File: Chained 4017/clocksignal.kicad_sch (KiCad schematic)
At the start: 6 parts, among them SW201 SW_Push, U201 LM555xM

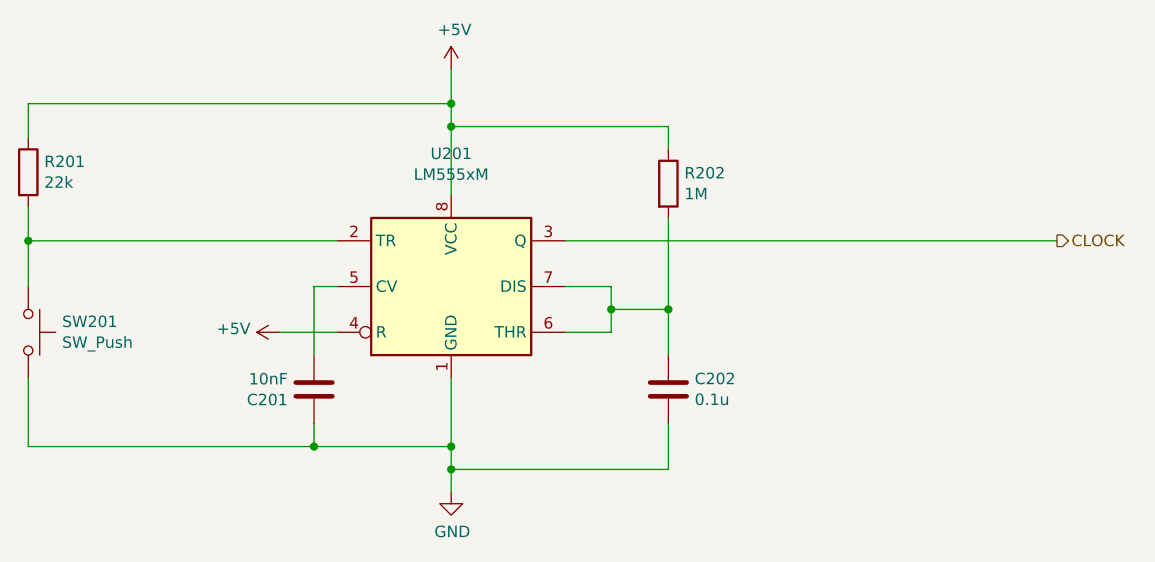
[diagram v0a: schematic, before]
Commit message: Complete routing
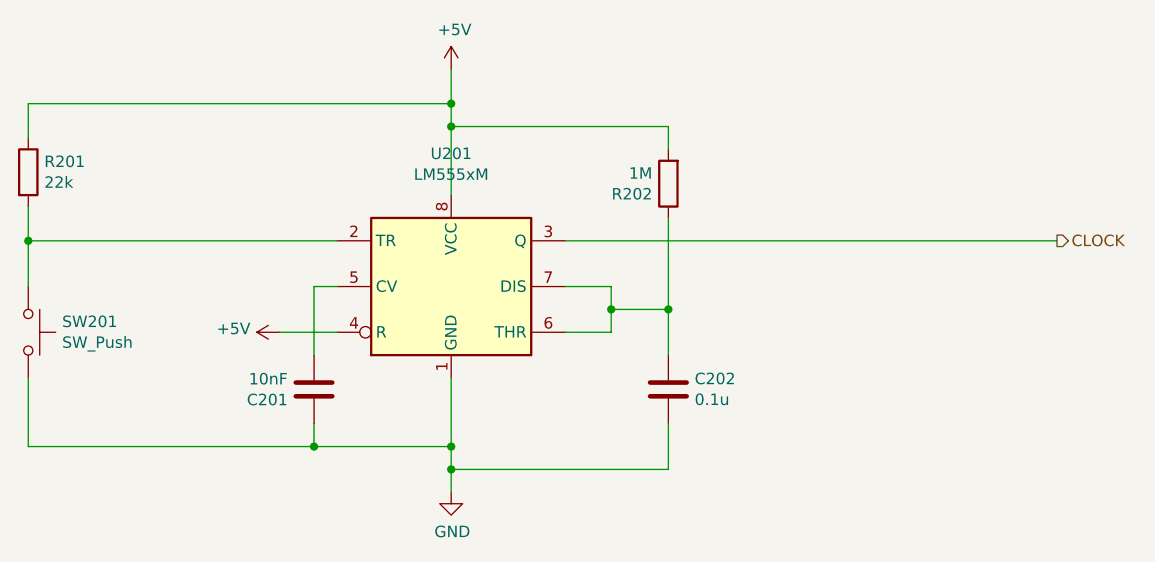
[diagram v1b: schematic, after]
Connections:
- net +5V: now also R202.2; no longer R202.1
- net at C202.1, U201.6 (THR), U201.7 (DIS): now also R202.1; no longer R202.2
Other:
- moved on the sheet: R202
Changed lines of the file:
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@@
     )
   )
-  (symbol (lib_id "Device:R") (at 121.92 67.31 0) (unit 1)
+  (symbol (lib_id "Device:R") (at 121.92 67.31 180) (unit 1)
     (in_bom yes) (on_board yes) (dnp no)
-    (property "Reference" "R202" (at 123.698 66.1416 0)
+    (property "Reference" "R202" (at 120.142 68.4784 0)
       (effects (font (size 1.27 1.27)) (justify left))
     )
-    (property "Value" "1M" (at 123.698 68.453 0)
+    (property "Value" "1M" (at 120.142 66.167 0)
       (effects (font (size 1.27 1.27)) (justify left))
     )
-    (property "Footprint" "Resistor_THT:R_Axial_DIN0207_L6.3mm_D2.5mm_P7.62mm_Horizontal" (at 120.142 67.31 90)
+    (property "Footprint" "Resistor_THT:R_Axial_DIN0207_L6.3mm_D2.5mm_P7.62mm_Horizontal" (at 123.698 67.31 90)
       (effects (font (size 1.27 1.27)) hide)
     )
